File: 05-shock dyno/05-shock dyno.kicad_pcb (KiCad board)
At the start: 4 copper layers, 101.5 x 89.2 mm, 63 parts, among them IC1 ADS131M04IPWR, IC2 OPA320AIDBVR, IC3 SPX3819S-L_TR, J1 Conn_01x03, J2 RJ45, J3 XT30PW-M, J4 Conn_01x04, T1 749013011, U1 Teensy4.1, U2 REF5025ID, U3 AD5626BRMZ, U4 INA827AIDGK

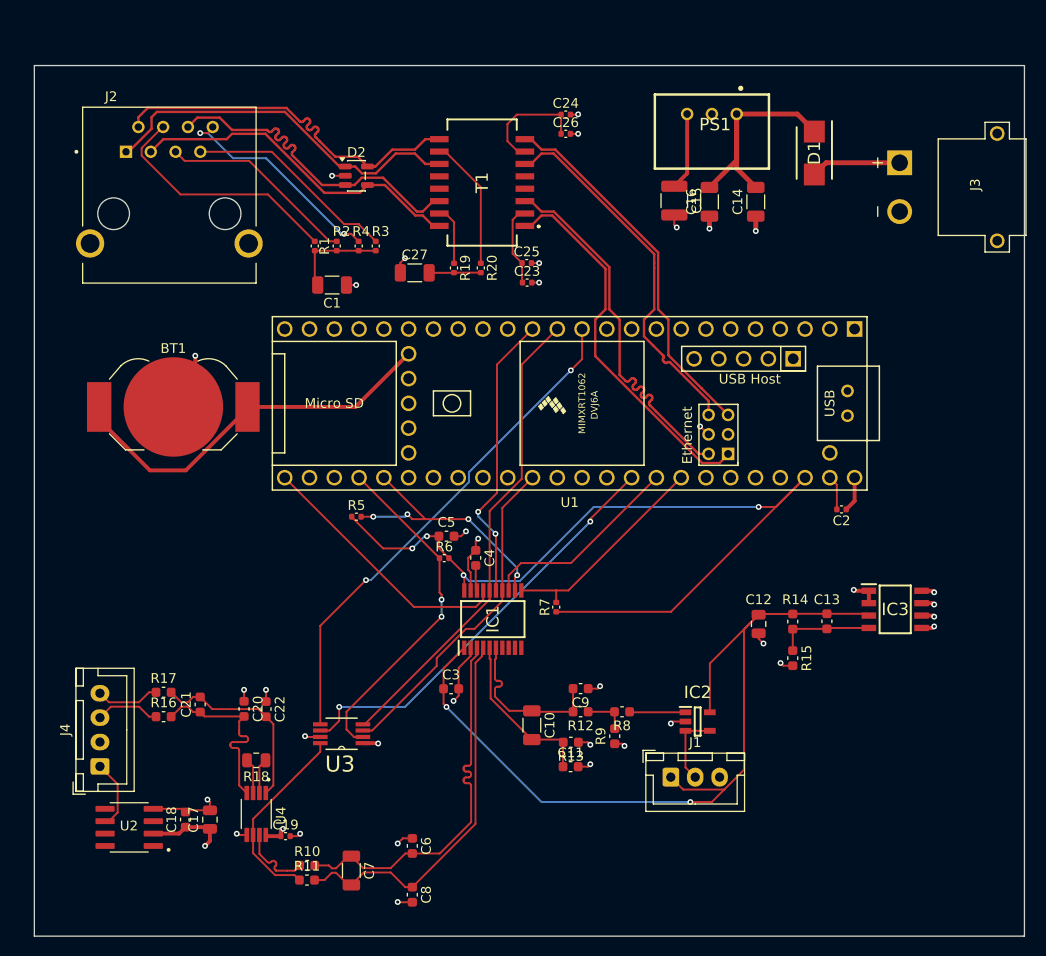
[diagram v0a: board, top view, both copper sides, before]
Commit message: v2 layout
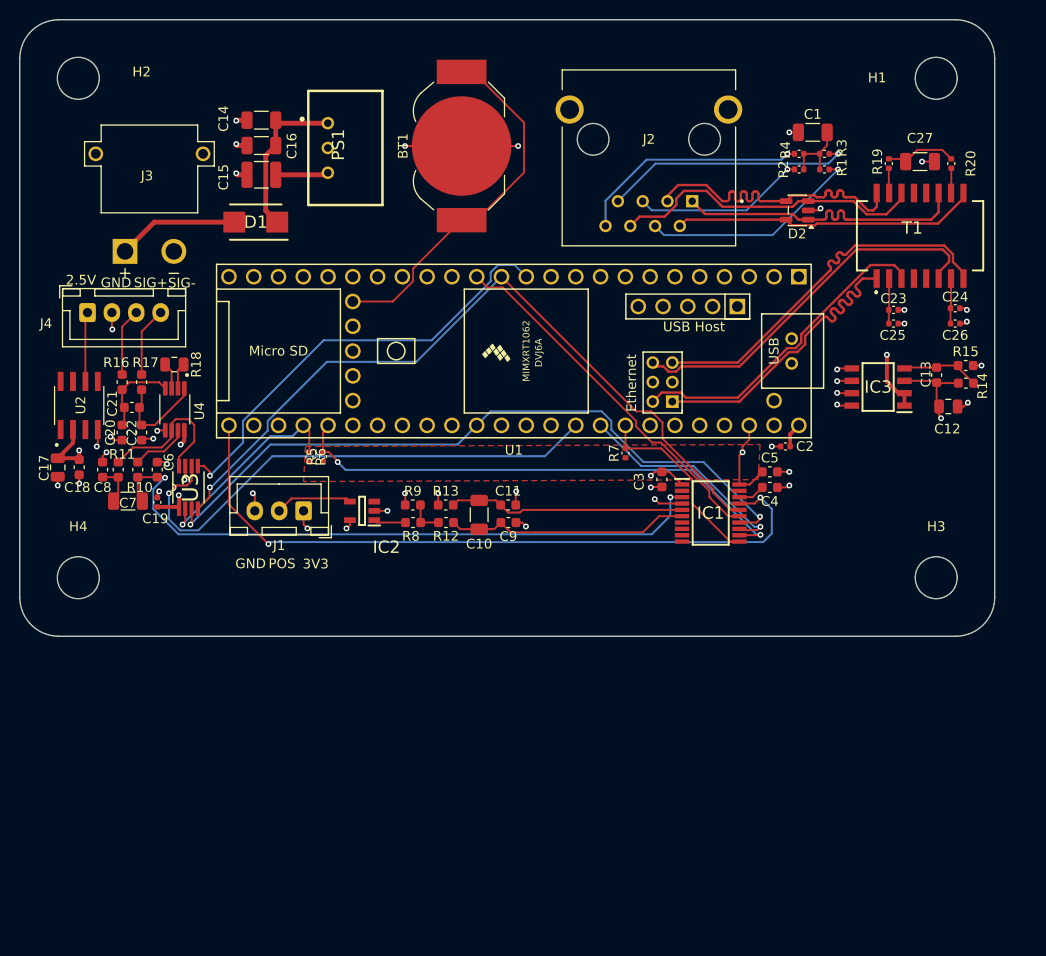
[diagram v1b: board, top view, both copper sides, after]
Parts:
- added G***: BJR_LOGO, 22XT_Main:BJR_LOGO, B.Cu at (140.2, 45.4)
- added H1: MountingHole_Pad, MountingHole:MountingHole_4.3mm_M4, F.Cu at (148.5, 47.1)
- added H2: MountingHole_Pad, MountingHole:MountingHole_4.3mm_M4, F.Cu at (60.5, 47.1)
- added H3: MountingHole_Pad, MountingHole:MountingHole_4.3mm_M4, F.Cu at (148.5, 98.3)
- added H4: MountingHole_Pad, MountingHole:MountingHole_4.3mm_M4, F.Cu at (60.5, 98.3)
- moved J3 87.0 mm to (67.8, 54.8), turned to 0 degrees
- moved D1 57.7 mm to (78.7, 61.8), turned to 180 degrees
- moved C8 53.9 mm to (63.0, 87.2), turned to 90 degrees
- moved C27 53.0 mm to (146.8, 55.6), turned to 180 degrees
- moved R1 52.8 mm to (137.0, 56.4), turned to 0 degrees
- moved C1 51.7 mm to (135.8, 52.6), turned to 0 degrees
- moved C14 51.4 mm to (79.3, 51.4), turned to 0 degrees
- moved J2 49.7 mm to (119.0, 53.3), turned to 180 degrees
- moved R20 49.4 mm to (150.0, 55.8), turned to 90 degrees
- moved R2 48.0 mm to (134.4, 56.4), turned to 180 degrees
- moved R3 47.0 mm to (137.0, 54.8), turned to 0 degrees
- moved C6 46.6 mm to (68.6, 87.2)
- moved J4 46.5 mm to (61.5, 71.1), turned to 0 degrees
- moved J1 46.5 mm to (83.6, 91.4), turned to 180 degrees
- moved R11 46.3 mm to (64.6, 87.2), turned to -90 degrees
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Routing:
- net 3v3_teensy: track 88.3 -> 9.37 mm, vias 4 -> 1
- net 3v3: track 89.0 -> 16.3 mm, vias 2 -> 4
- net ADC_CLK: track 27.1 -> 72.5 mm, vias 0 -> 2
- net SCLK1: track 34.2 -> 72.4 mm, vias 0 -> 2
- net amp_ref_nyq-: track 39.6 -> 7.23 mm, vias 0 -> 1
- net MOSI1: track 48.9 -> 77.6 mm, vias 0 -> 1
- net amp_ref_nyq+: track 39.4 -> 67.2 mm, vias 0 -> 2
- net CS_ADC: track 26.8 -> 53.5 mm, vias 4 -> 2
- net CS_DAC: track 35.9 -> 21.4 mm, vias 2 -> 1
- net GND: track 67.1 -> 55.4 mm, vias 34 -> 39
- net Net-(T1-TXCT): track 13.6 -> 2.55 mm
- net loadcell_f+: track 19.6 -> 8.81 mm
- net CLR_DAC: track 43.6 -> 53.7 mm, vias 2 -> 1
- net loadcell_f-: track 19.7 -> 10.2 mm
- net 11.1V: track 25.8 -> 17.0 mm
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- added copper zone on In2.Cu, net 3v3
- added copper zone on F.Cu, net 3v3_teensy
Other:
- board size 101.5 x 89.2 mm -> 100 x 63.2 mm
- board text added: "2.5V"
- board text added: "3V3"
- board text added: "Blue Jay Racing @ JHU 23XT Shock Dyno V1"
- board text added: "GND"
- board text added: "Max Gao"
- board text added: "POS"
- board text added: "SIG+"
- board text added: "SIG-"
- board text added: "Sophie Noureddine"
